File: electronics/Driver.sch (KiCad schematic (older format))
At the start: 27 parts

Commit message: Another restructure, added CPU pins, updated V regulators
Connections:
- wire segments 69 -> 57
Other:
- note added: "Motor 1 driver"
- note added: "Motor 2 driver"
- note added: "Motor 3 driver"
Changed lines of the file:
@@
 $Descr A4 11693 8268
 encoding utf-8
-Sheet 3 5
+Sheet 2 3
 Title ""
 Date ""
@@
 Wire Wire Line
 	1750 2800 1750 2900
-Text Label 1400 1900 0    50   ~ 0
-MOT1en_2
-Text Label 1400 1800 0    50   ~ 0
-MOT1en_1
 $Comp
 L Device:R_US R?
@@
 	1    0    0    -1
 $EndComp
-Wire Wire Line
-	1400 1800 1850 1800
-Wire Wire Line
-	1400 1900 1850 1900
 $Comp
 L Device:C C?
@@
 Wire Wire Line
 	5400 2800 5400 2900
-Text Label 5050 1900 0    50   ~ 0
-MOT2en_2
-Text Label 5050 1800 0    50   ~ 0
-MOT2en_1
 $Comp
 L Device:R_US R?
@@
 	1    0    0    -1
 $EndComp
-Wire Wire Line
-	5050 1800 5500 1800
-Wire Wire Line
-	5050 1900 5500 1900
 $Comp
 L Device:C C?
@@
 Wire Wire Line
 	8850 2800 8850 2900
-Wire Wire Line
-	8500 2200 8950 2200
-Text Label 8500 2200 0    50   ~ 0
-MOT_off
-Wire Wire Line
-	8500 2000 8950 2000
-Text Label 8500 2000 0    50   ~ 0
-MOT_sleep
-Text Label 8500 1900 0    50   ~ 0
-MOT3en_2
 $Comp
 L Device:R_US R?
@@
 	1    0    0    -1
 $EndComp
-Wire Wire Line
-	8500 1800 8950 1800
-Wire Wire Line
-	8500 1900 8950 1900
 $Comp
 L power:Earth #PWR0131
@@
 Connection ~ 9950 2100
 Connection ~ 9950 2400
-Wire Wire Line
-	5050 2200 5500 2200
-Text Label 5050 2200 0    50   ~ 0
+Text HLabel 8950 1800 0    50   Input ~ 0
+MOT3en_1
+Text HLabel 8950 1900 0    50   Input ~ 0
+MOT3en_2
+Text HLabel 8950 2000 0    50   Input ~ 0
+MOT_sleep
+Text HLabel 8950 2200 0    50   Input ~ 0
 MOT_off
-Wire Wire Line
-	5050 2000 5500 2000
-Text Label 5050 2000 0    50   ~ 0
+Text HLabel 1850 1800 0    50   Input ~ 0
+MOT1en_1
+Text HLabel 1850 1900 0    50   Input ~ 0
+MOT1en_2
+Text HLabel 5500 1800 0    50   Input ~ 0
+MOT2en_1
+Text HLabel 5500 1900 0    50   Input ~ 0
+MOT2en_2
+Text HLabel 5500 2000 0    50   Input ~ 0
 MOT_sleep
-Wire Wire Line
-	1400 2200 1850 2200
-Text Label 1400 2200 0    50   ~ 0
+Text HLabel 5500 2200 0    50   Input ~ 0
 MOT_off
-Wire Wire Line
-	1400 2000 1850 2000
-Text Label 1400 2000 0    50   ~ 0
+Text HLabel 1850 2000 0    50   Input ~ 0
 MOT_sleep
-Text HLabel 8500 1800 0    50   Input ~ 0
-MOT3en_1
+Text HLabel 1850 2200 0    50   Input ~ 0
+MOT_off
+Text Notes 2050 3450 0    50   ~ 0
+Motor 1 driver
+Text Notes 5700 3500 0    50   ~ 0
+Motor 2 driver
+Text Notes 9250 3450 0    50   ~ 0
+Motor 3 driver
 $EndSCHEMATC

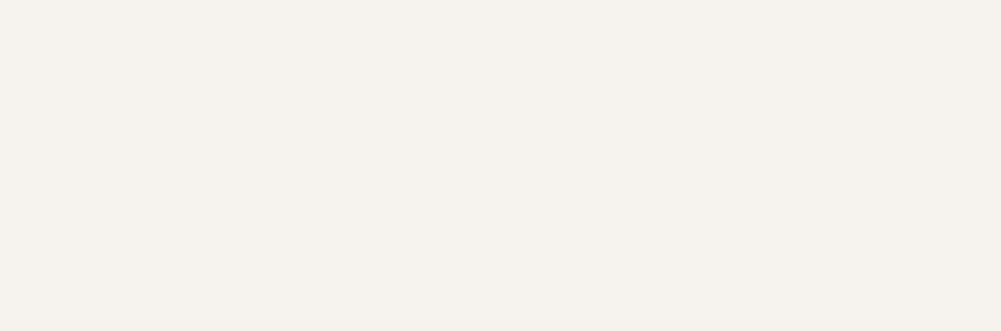
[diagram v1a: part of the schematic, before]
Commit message: Updated titles
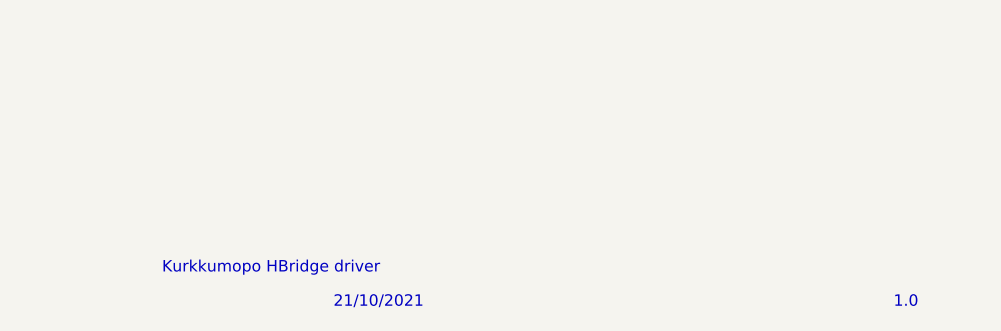
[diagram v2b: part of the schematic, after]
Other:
- note added: "1.0"
- note added: "21/10/2021"
- note added: "Kurkkumopo HBridge driver"
